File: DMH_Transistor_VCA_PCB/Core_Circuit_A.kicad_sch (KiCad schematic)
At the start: 28 parts, among them Q1 BC548, Q2 BC548, U1 TL074

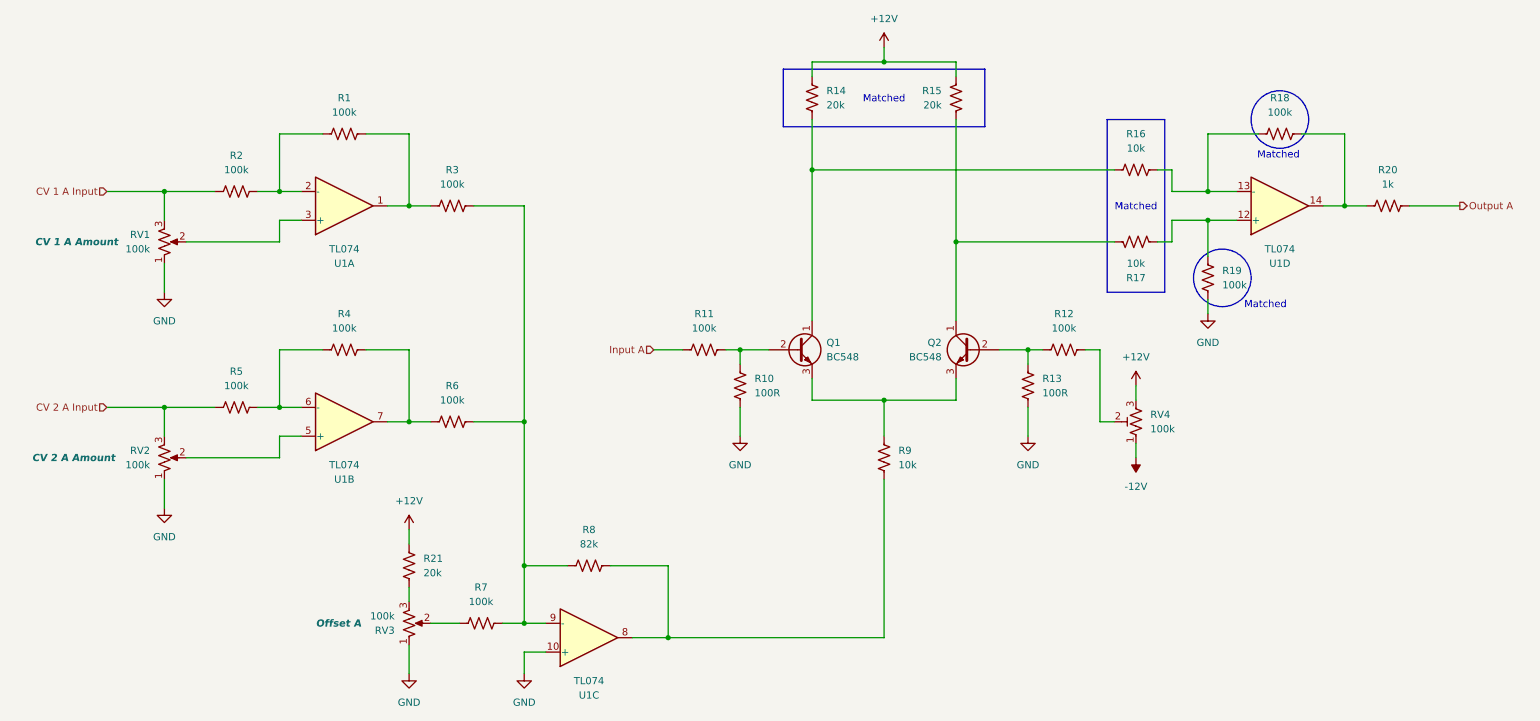
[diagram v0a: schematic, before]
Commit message: Finished schematic
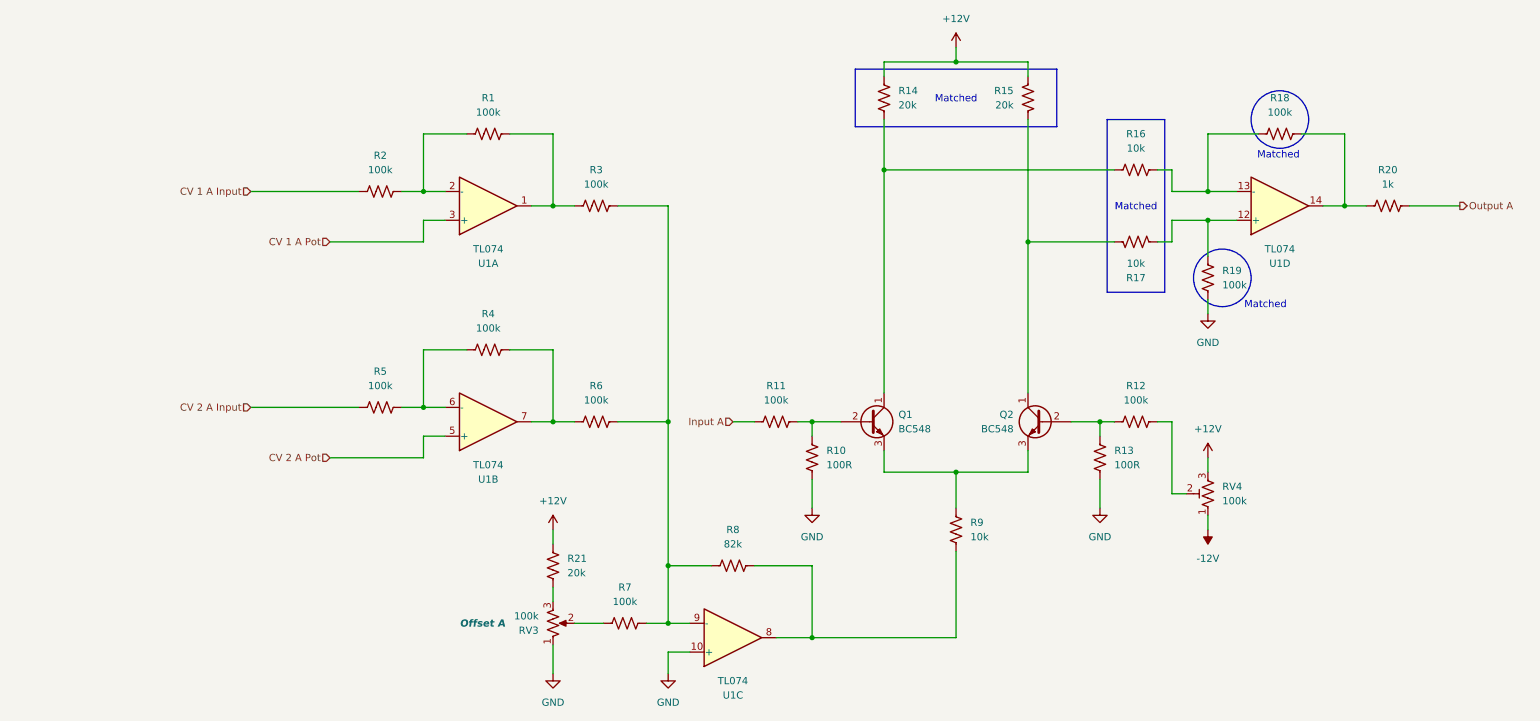
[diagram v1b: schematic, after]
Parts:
- removed RV1, RV2: 100k, SynthStuff:Potentiometer_TT_P110KH1, symbol Device:R_Potentiometer_US
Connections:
- net CV 1 A Pot: now reaches U1.3 (+)
- net CV 2 A Pot: now reaches U1.5 (+)
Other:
- moved on the sheet: Q1, Q2, R1, R10, R11, R12, R13, R14, R15, R2, R21, R3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
